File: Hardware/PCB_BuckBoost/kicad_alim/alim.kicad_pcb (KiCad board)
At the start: 2 copper layers, 41 x 67.3 mm, 36 parts, among them J1 Conn_01x02, J2 Conn_01x02, J3 Conn_01x02, J4 Conn_01x02, U1 MIC3172YM, U2 MIC3172YM

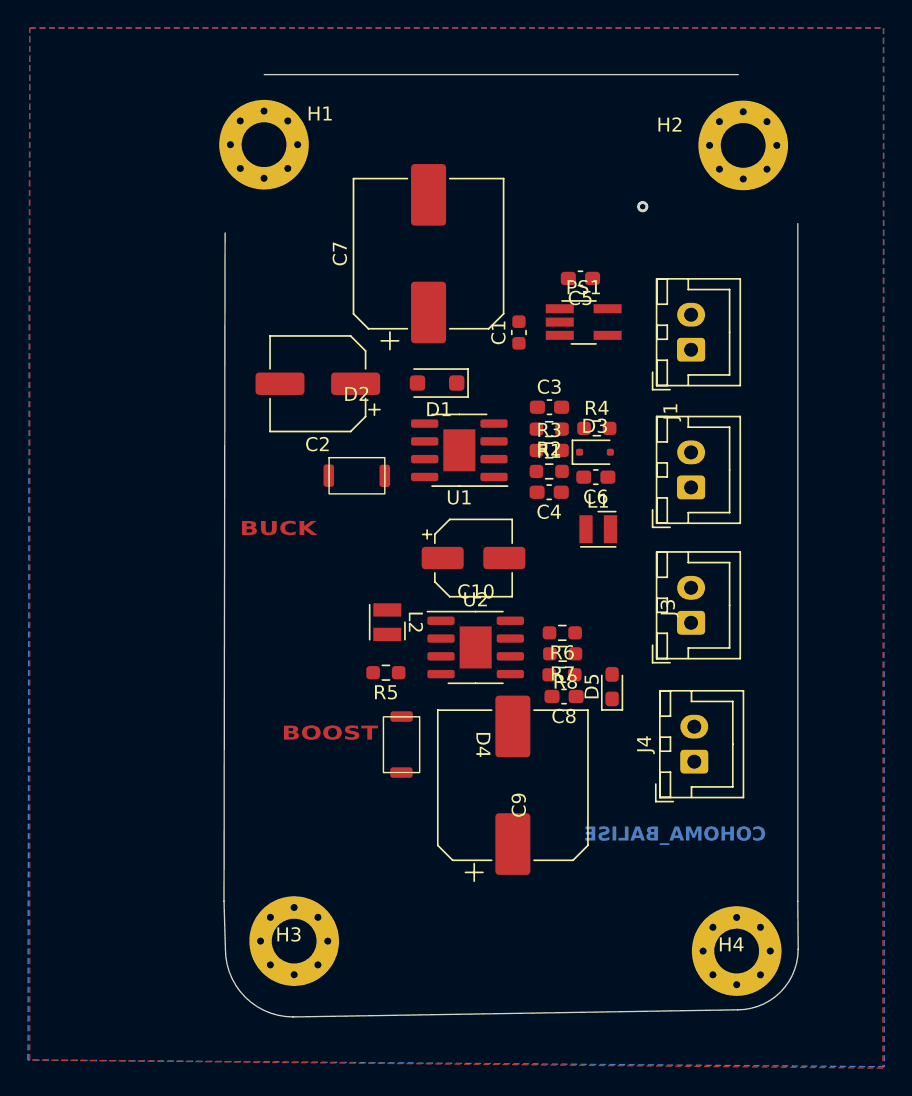
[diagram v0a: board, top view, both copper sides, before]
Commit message: a
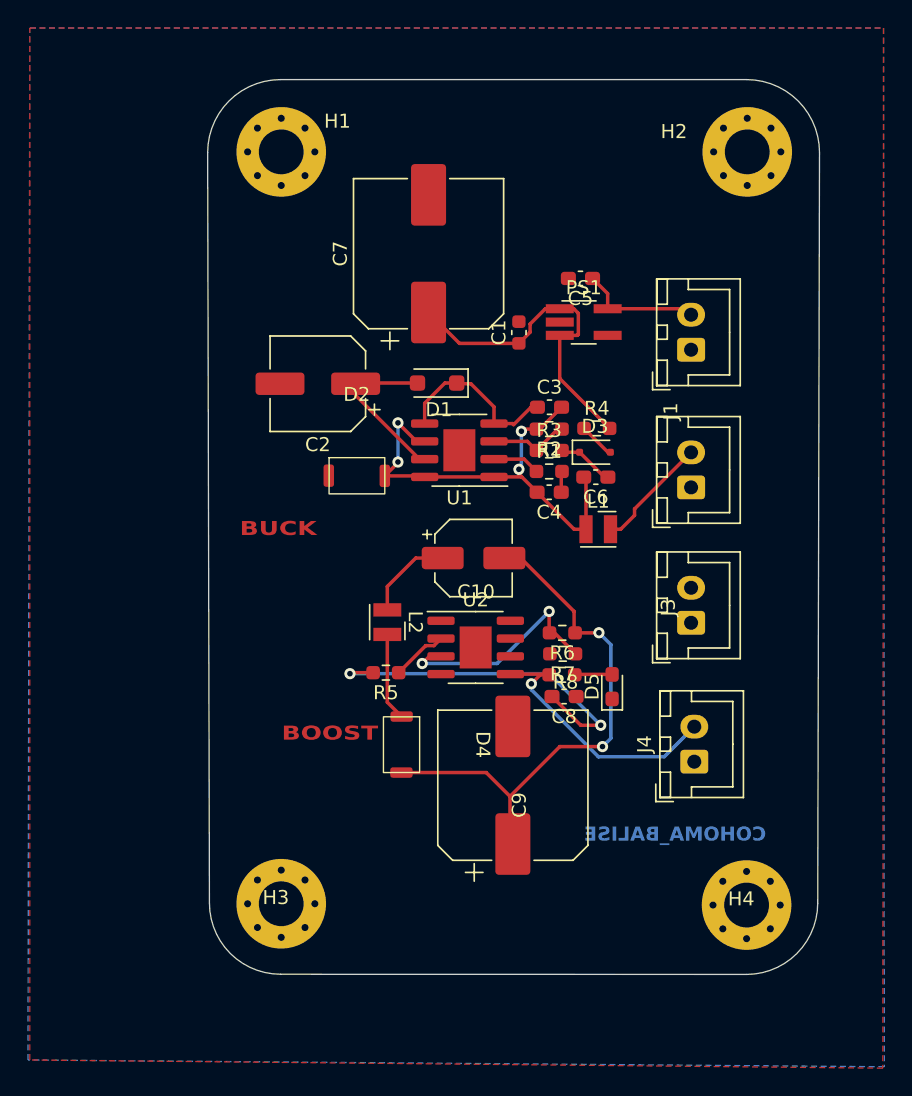
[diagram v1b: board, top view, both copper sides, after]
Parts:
- moved H4 3.36 mm to (197.2, 127.4)
- moved H3 2.82 mm to (164.0, 127.3)
- moved H1 1.33 mm to (164.0, 73.6)
- moved H2 0.54 mm to (197.3, 73.6)
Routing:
- net Routeur: track 0.00 -> 38.6 mm, vias 0 -> 2
- net +15V: track 0.00 -> 37.8 mm, vias 0 -> 1
- net Net-(D2-K): track 0.00 -> 33.4 mm, vias 0 -> 4
- net +5V: track 0.00 -> 32.4 mm
- net Net-(C8-Pad2): track 0.00 -> 25.4 mm, vias 0 -> 2
- net Net-(U2-FB): track 0.00 -> 16.2 mm, vias 0 -> 2
- net Net-(D1-K): track 0.00 -> 12.5 mm
- net +3.3V: track 0.00 -> 8.75 mm, vias 1 -> 0
- net Net-(D4-A): track 0.00 -> 6.29 mm
- net Net-(U1-FB): track 0.00 -> 5.75 mm
- net Net-(D3-K): track 0.00 -> 4.07 mm
- net Net-(U2-COMP): track 0.00 -> 4.03 mm
- net Net-(U1-COMP): track 0.00 -> 3.39 mm
- net Net-(D5-A): track 0.00 -> 2.68 mm
- net Net-(D3-A): track 0.00 -> 2.58 mm
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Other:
- board size 41 x 67.3 mm -> 43.7 x 63.9 mm
